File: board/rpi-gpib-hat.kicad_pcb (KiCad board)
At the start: 2 copper layers, 65 x 30 mm, 44 parts, among them J1 RPI_GPIO, J2 GPIB, U1 SN75160BDW, U2 SN75162BDW, U3 LM317_SOT-223, U4 CAT24C32

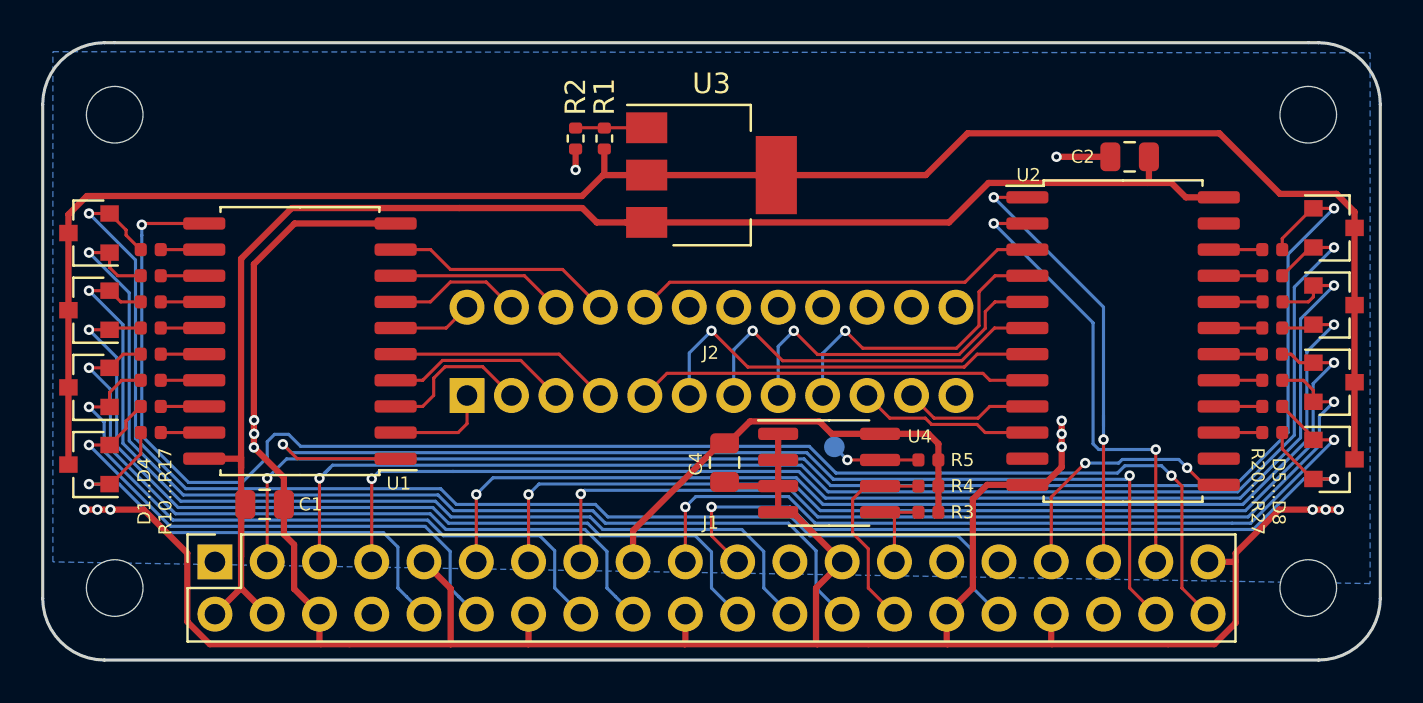
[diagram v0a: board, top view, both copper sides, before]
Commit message: Clean up routing.
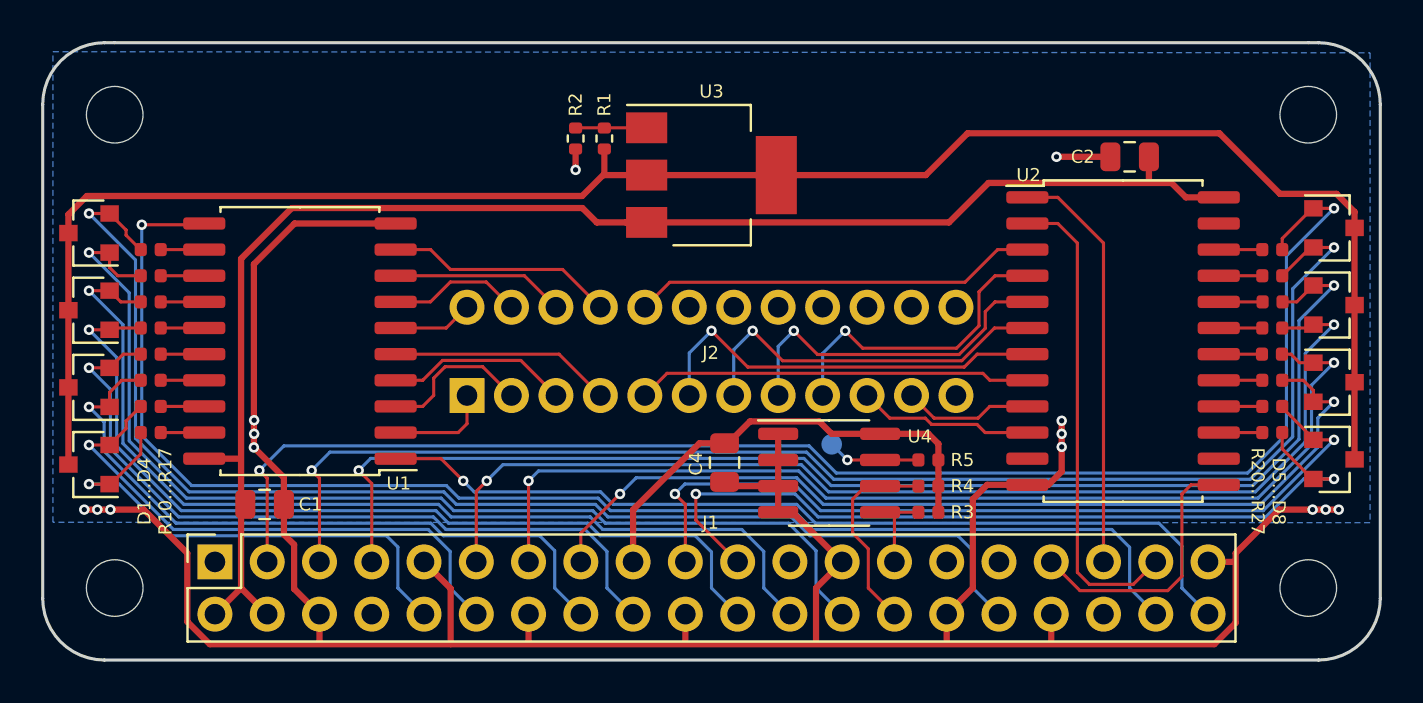
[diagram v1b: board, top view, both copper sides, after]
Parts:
- moved TP1 0.18 mm to (134.8, 116.0)
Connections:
- U1 pad 1: /GPIO20 -> /GPIO21
- U1 pad 11: /GPIO21 -> /GPIO20
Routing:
- net /GPIO21: track 74.3 -> 43.8 mm, vias 2 -> 1
- net /GPIO20: track 55.0 -> 67.3 mm, vias 2 -> 1
- net /GPIO24: track 36.9 -> 43.5 mm
- net +5V: track 77.1 -> 74.1 mm
- net /GPIO19: track 22.1 -> 20.1 mm, vias 2 -> 0
- net /GPIO9: track 38.8 -> 40.3 mm
- net /GPIO22: track 46.9 -> 45.8 mm
- net /GPIO10: track 39.9 -> 41.0 mm
- net /GPIO2: track 71.1 -> 71.9 mm
- net /GPIO4: track 62.4 -> 63.1 mm
- net /GPIO13: track 12.6 -> 13.2 mm, vias 2 -> 0
- net +3V3: track 22.3 -> 22.9 mm
- net /GPIO26: track 23.1 -> 23.3 mm, vias 2 -> 0
